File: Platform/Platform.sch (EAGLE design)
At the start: 38 parts, among them J1 DC21MMX, U1 FT232RLSSOP, X1 USBSMD, Y1 RESONATORSMD

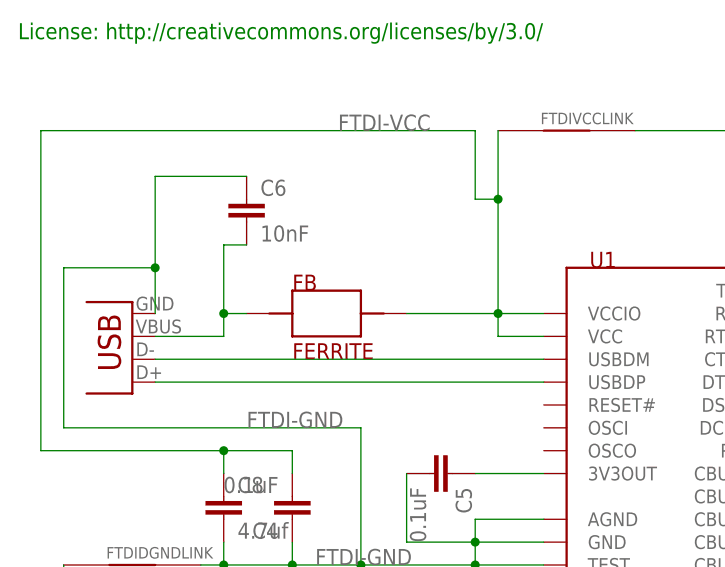
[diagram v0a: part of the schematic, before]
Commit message: Final Design for Production
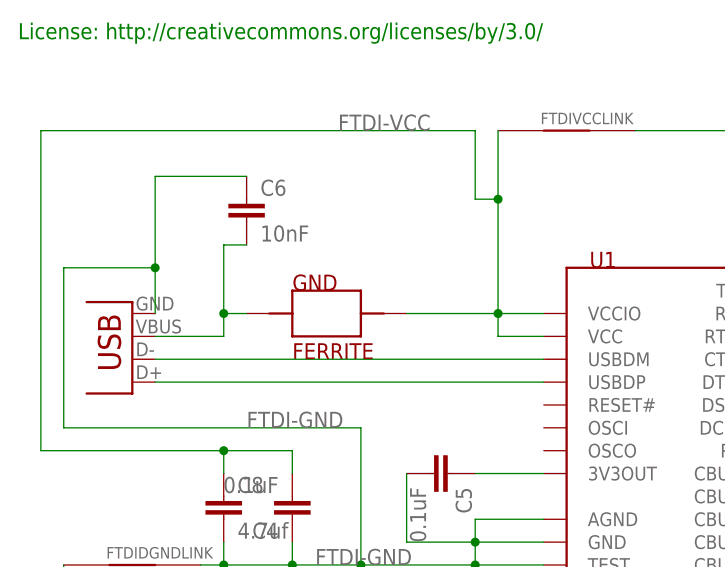
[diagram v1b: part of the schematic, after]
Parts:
- renumbered FB to GND
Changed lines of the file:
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@@
 <?xml version="1.0" encoding="utf-8"?>
 <!DOCTYPE eagle SYSTEM "eagle.dtd">
-<eagle version="6.2">
+<eagle version="6.1">
 <drawing>
 <settings>
@@
 <attribute name="DIGIKEY#" value="768-1007-1-ND"/>
 </part>
-<part name="FB" library="Dustin" deviceset="FERRITE" device="">
+<part name="GND" library="Dustin" deviceset="FERRITE" device="">
 <attribute name="DIGIKEY#" value="240-2399-1-ND"/>
 </part>
@@
 <attribute name="DIGIKEY#" x="66.04" y="134.62" size="1.778" layer="96" display="off"/>
 </instance>
-<instance part="FB" gate="G$1" x="27.94" y="149.86">
+<instance part="GND" gate="G$1" x="27.94" y="149.86">
 <attribute name="DIGIKEY#" x="27.94" y="149.86" size="1.778" layer="96" display="off"/>
 </instance>
@@
 <wire x1="10.16" y1="147.32" x2="17.78" y2="147.32" width="0.1524" layer="91"/>
 <wire x1="17.78" y1="147.32" x2="17.78" y2="149.86" width="0.1524" layer="91"/>
-<pinref part="FB" gate="G$1" pin="P$1"/>
+<pinref part="GND" gate="G$1" pin="P$1"/>
 <wire x1="17.78" y1="149.86" x2="20.32" y2="149.86" width="0.1524" layer="91"/>
 <junction x="17.78" y="149.86"/>
@@
 <net name="FTDI-VCC" class="0">
 <segment>
-<pinref part="FB" gate="G$1" pin="P$2"/>
+<pinref part="GND" gate="G$1" pin="P$2"/>
 <wire x1="38.1" y1="149.86" x2="48.26" y2="149.86" width="0.1524" layer="91"/>
 <junction x="48.26" y="149.86"/>
